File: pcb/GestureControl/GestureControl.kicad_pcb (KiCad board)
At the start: 4 copper layers, 95.3 x 87.6 mm, 102 parts, among them J1 Conn_01x04_I2I-LCD, J10 EXTERN I2C, J11 Conn_01x01, J12 Conn_01x01, J13 Conn_01x01, J14 Conn_01x01, J15 Conn_01x01, J16 Conn_01x01, J17 Conn_01x01, J18 Conn_01x01, J19 Conn_01x01, J2 BATT, J3 Conn_01x08, J4 Conn_01x06, J5 Conn_01x10, J6 Conn_01x08, J7 FTDI, J8 Serial Wire, J9 UART, SW1 SW1, SW2 SW2, SW3 BOOT, SW4 RST, U1 LD1117-3.3, U2 LD1117-5.0, U3 VL53L3CXV0DH_CENTER, U4 VL53L3CXV0DH_RIGHT, U5 VL53L3CXV0DH_LEFT, U6 STM32L151RETx, U7 STM32F401RETx, Y1 8MHz, Y2 32kHz

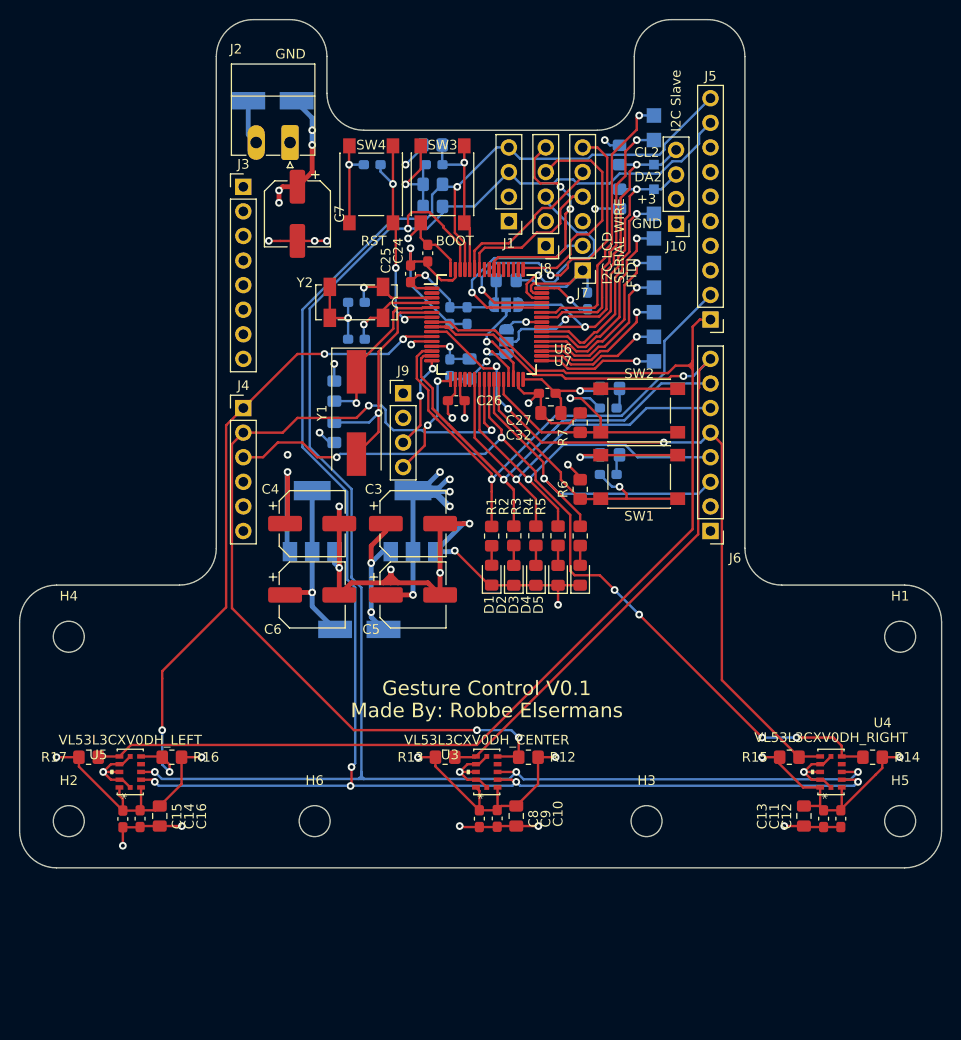
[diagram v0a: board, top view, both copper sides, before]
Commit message: add feedback Philip
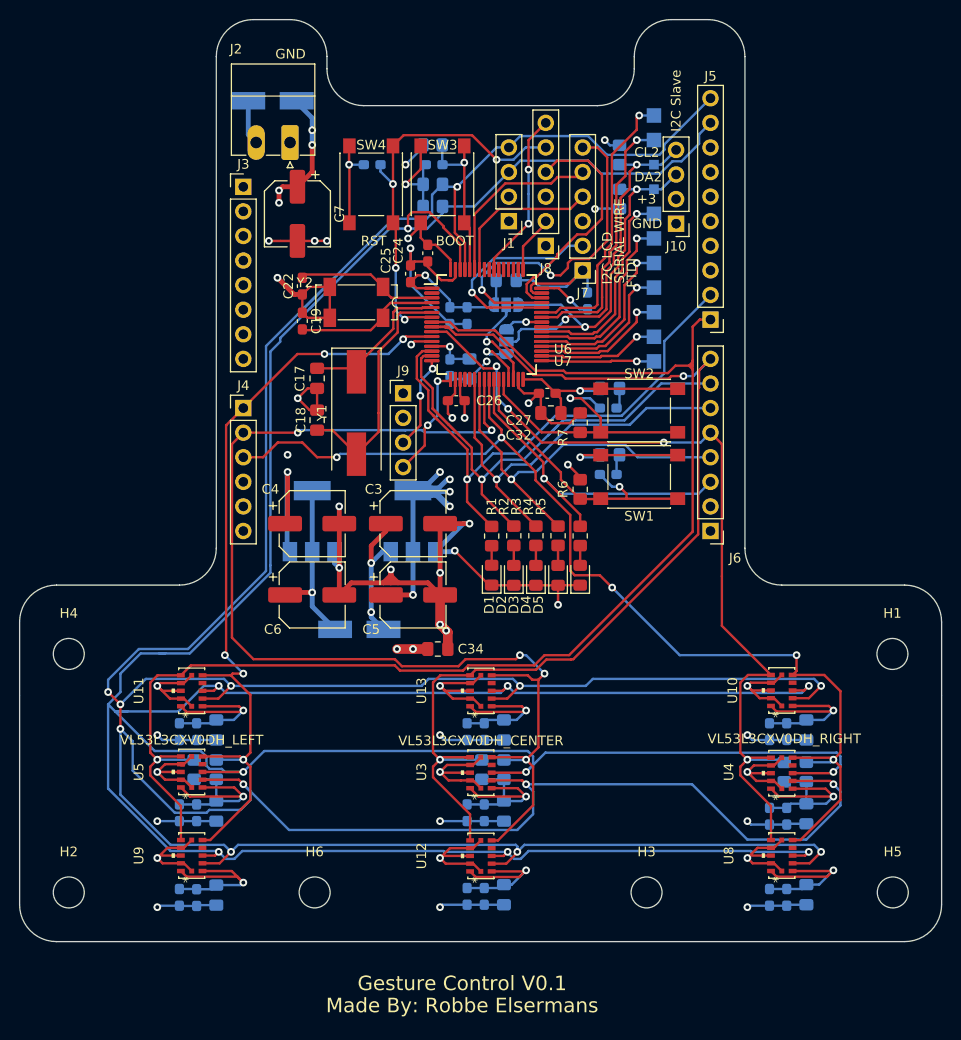
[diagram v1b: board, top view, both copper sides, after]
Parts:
- added C34: 4.7µ, Capacitor_SMD:C_0805_2012Metric_Pad1.18x1.45mm_HandSolder, F.Cu at (142.0, 102.9)
- added C35: 100n, Capacitor_SMD:C_0603_1608Metric_Pad1.08x0.95mm_HandSolder, B.Cu at (146.8, 111.4)
- added C36: 100n, Capacitor_SMD:C_0603_1608Metric_Pad1.08x0.95mm_HandSolder, B.Cu at (146.8, 128.4)
- added C37: 4.7µ, Capacitor_SMD:C_0805_2012Metric_Pad1.18x1.45mm_HandSolder, B.Cu at (148.8, 111.2)
- added C38: 4.7µ, Capacitor_SMD:C_0805_2012Metric_Pad1.18x1.45mm_HandSolder, B.Cu at (148.8, 128.2)
- added C39: 100n, Capacitor_SMD:C_0603_1608Metric_Pad1.08x0.95mm_HandSolder, B.Cu at (178.1, 128.5)
- added C40: 100n, Capacitor_SMD:C_0603_1608Metric_Pad1.08x0.95mm_HandSolder, B.Cu at (176.3, 111.4)
- added C41: 4.7µ, Capacitor_SMD:C_0805_2012Metric_Pad1.18x1.45mm_HandSolder, B.Cu at (180.1, 128.2)
- added C42: 4.7µ, Capacitor_SMD:C_0805_2012Metric_Pad1.18x1.45mm_HandSolder, B.Cu at (180.1, 111.2)
- added C43: 100n, Capacitor_SMD:C_0603_1608Metric_Pad1.08x0.95mm_HandSolder, B.Cu at (115.3, 128.5)
- added C44: 100n, Capacitor_SMD:C_0603_1608Metric_Pad1.08x0.95mm_HandSolder, B.Cu at (115.3, 111.4)
- added C45: 4.7µ, Capacitor_SMD:C_0805_2012Metric_Pad1.18x1.45mm_HandSolder, B.Cu at (119.1, 128.3)
- added C46: 4.7µ, Capacitor_SMD:C_0805_2012Metric_Pad1.18x1.45mm_HandSolder, B.Cu at (119.1, 111.2)
- added C47: 100n, Capacitor_SMD:C_0603_1608Metric_Pad1.08x0.95mm_HandSolder, B.Cu at (145.0, 111.4)
- added C48: 100n, Capacitor_SMD:C_0603_1608Metric_Pad1.08x0.95mm_HandSolder, B.Cu at (145.0, 128.4)
- added C49: 100n, Capacitor_SMD:C_0603_1608Metric_Pad1.08x0.95mm_HandSolder, B.Cu at (178.1, 111.4)
- added C50: 100n, Capacitor_SMD:C_0603_1608Metric_Pad1.08x0.95mm_HandSolder, B.Cu at (176.3, 128.5)
- added C51: 100n, Capacitor_SMD:C_0603_1608Metric_Pad1.08x0.95mm_HandSolder, B.Cu at (117.1, 111.4)
- added C52: 100n, Capacitor_SMD:C_0603_1608Metric_Pad1.08x0.95mm_HandSolder, B.Cu at (117.1, 128.6)
- added U10: VL53L3CXV0DH_RIGHT, VL53L3CX:VL53L3CXV0DH&slash_1, F.Cu at (177.5, 107.1)
- added U11: VL53L3CXV0DH_LEFT, VL53L3CX:VL53L3CXV0DH&slash_1, F.Cu at (116.6, 107.2)
- added U12: VL53L3CXV0DH_CENTER, VL53L3CX:VL53L3CXV0DH&slash_1, F.Cu at (146.5, 124.2)
- added U13: VL53L3CXV0DH_CENTER, VL53L3CX:VL53L3CXV0DH&slash_1, F.Cu at (146.5, 107.2)
- added U8: VL53L3CXV0DH_RIGHT, VL53L3CX:VL53L3CXV0DH&slash_1, F.Cu at (177.5, 124.2)
- added U9: VL53L3CXV0DH_LEFT, VL53L3CX:VL53L3CXV0DH&slash_1, F.Cu at (116.6, 124.2)
- C10, C11, C12, C13, C14, C15, C16, C8, C9, R12, R13, R14, R15, R16, R17: moved to B.Cu
- C17, C18, C19, C22: moved to F.Cu
- J8: value Serial Wire -> Conn_01x06; footprint Connector_PinHeader_2.54mm:PinHeader_1x05_P2.54mm_Vertical -> Connector_PinHeader_2.54mm:PinHeader_1x06_P2.54mm_Vertical
- moved R17 11.0 mm to (116.8, 115.3), turned to 90 degrees
- moved H5 7.41 mm to (189.0, 128.0)
- moved C12 7.37 mm to (176.3, 120.1)
- moved H2 7.37 mm to (103.9, 128.0)
- moved H3 7.37 mm to (163.6, 128.0)
- moved H6 7.37 mm to (129.3, 128.0)
- moved R14 7.01 mm to (180.1, 115.6), turned to 90 degrees
- moved U5 6.35 mm to (116.6, 115.6)
- moved C19 5.90 mm to (128.0, 69.0), turned to 270 degrees
- moved C15 5.88 mm to (115.3, 119.8)
- moved C14 5.87 mm to (117.1, 119.8)
- moved C16 5.86 mm to (119.1, 119.6)
- moved C22 5.83 mm to (128.0, 65.4), turned to 90 degrees
- moved U4 5.08 mm to (177.5, 115.7)
- moved R16 4.76 mm to (119.1, 115.3), turned to 90 degrees
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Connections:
- J8 pad 1: GND -> +3V3
- J8 pad 2: +3V3 -> /STM32L151RET6TR/SWCLK
- J8 pad 3: /STM32L151RET6TR/SWDAT -> GND
- J8 pad 4: /STM32L151RET6TR/SWCLK -> /STM32L151RET6TR/SWDAT
- J8 pad 5: /STM32L151RET6TR/SW0 -> /STM32L151RET6TR/RST
- U3 pad 8: (no net) -> Net-(U12-Pad8)
- U4 pad 8: (no net) -> Net-(U10-Pad8)
- U5 pad 8: (no net) -> Net-(U11-Pad8)
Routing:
- net +3V3: track 506.8 -> 786.6 mm, vias 21 -> 26
- net SCL1: track 193.2 -> 410.9 mm, vias 6 -> 13
- net SDA1: track 194.0 -> 385.5 mm, vias 4 -> 10
- net GND: track 205.5 -> 343.5 mm, vias 29 -> 40
- net GPIOI_1: track 92.4 -> 121.2 mm, vias 4 -> 5
- net XSHUT_1: track 86.3 -> 112.0 mm, vias 1 -> 2
- net GPIOI_2: track 90.9 -> 113.3 mm, vias 6 -> 5
- net /STM32L151RET6TR/RST: track 23.9 -> 42.2 mm, vias 3 -> 4
- net /STM32L151RET6TR/SWCLK: track 22.9 -> 5.96 mm
- net XSHUT_0: track 124.9 -> 141.5 mm, vias 0 -> 1
- net XSHUT_2: track 75.5 -> 91.8 mm, vias 3 -> 4
- net GPIOI_0: track 68.0 -> 84.0 mm, vias 4 -> 5
- net LED_2: track 62.9 -> 55.6 mm
- net /STM32L151RET6TR/SW0: track 23.6 -> 17.4 mm
- net /STM32L151RET6TR/OS32_IN: track 9.26 -> 14.7 mm, vias 1 -> 0
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- added copper zone on PWR, net +3V3
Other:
- board size 95.3 x 87.6 mm -> 95.3 x 95.3 mm
